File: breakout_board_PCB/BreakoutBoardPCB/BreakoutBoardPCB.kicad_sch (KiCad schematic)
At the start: 16 parts, among them IC1 AD5676BRUZ, IC2 MCP3464T-E_NC, IC3 23K256T-I_SN, IC4 23K256T-I_SN, IC5 23K256T-I_SN, IC6 23K256T-I_SN, IC7 MCP3464T-E_NC, J1 SJ-63062A, J10 Conn_01x27_Female, J11 Conn_01x20_Female, J2 SJ-63062A, J7 Conn_01x06_Female

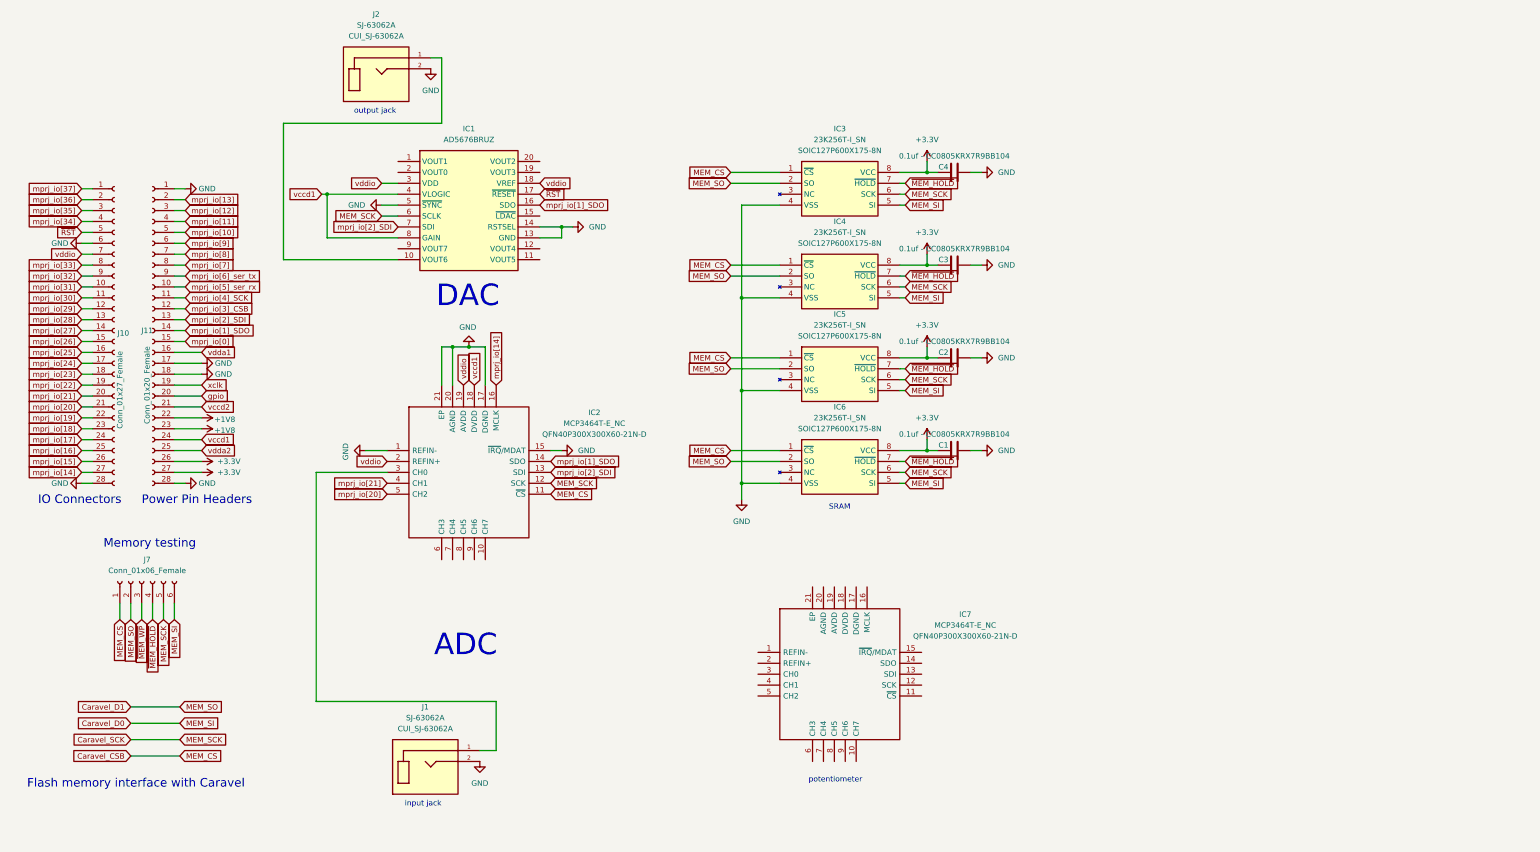
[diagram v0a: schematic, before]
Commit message: update 4/5
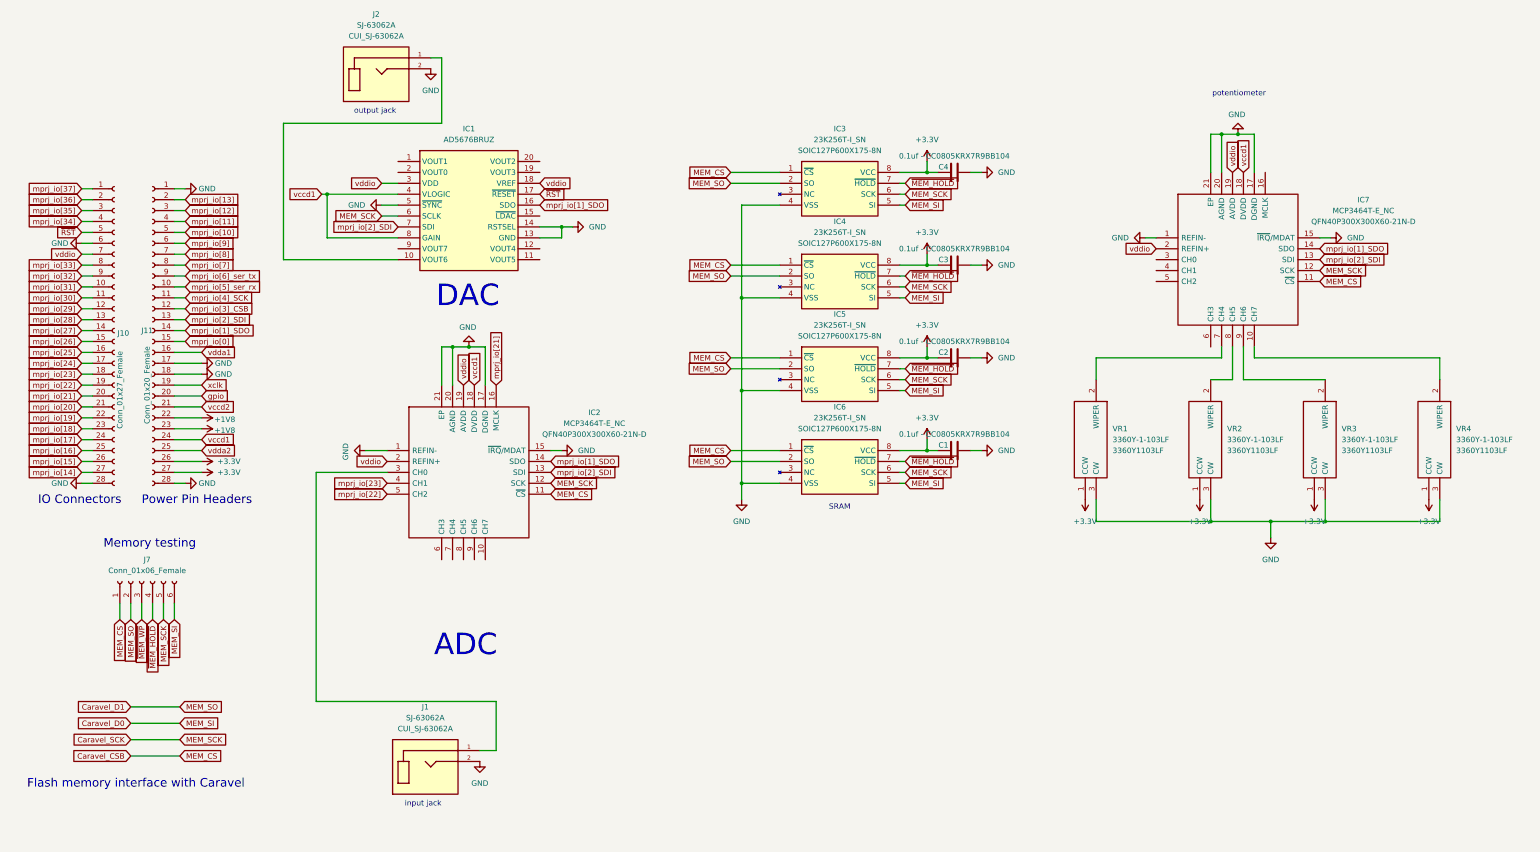
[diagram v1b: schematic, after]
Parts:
- added VR1, VR2, VR3, VR4: 3360Y-1-103LF, 3360Y1103LF, symbol SeniorDesign:3360Y-1-103LF
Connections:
- net +3.3V: now also VR1.1 (CCW), VR2.1 (CCW), VR3.1 (CCW), VR4.1 (CCW)
- net Caravel_CSB: now also IC7.11 (~{CS})
- net Caravel_SCK: now also IC7.12 (SCK)
- net GND: now also IC7.1 (REFIN-), IC7.15 (~{IRQ}/MDAT), IC7.17 (DGND), IC7.20 (AGND), IC7.21 (EP), VR1.3 (CW), VR2.3 (CW), VR3.3 (CW), VR4.3 (CW)
- net mprj_io[14]: no longer IC2.16 (MCLK)
- net mprj_io[1]_SDO: now also IC7.14 (SDO)
- net mprj_io[20]: no longer IC2.5 (CH2)
- net mprj_io[21]: now also IC2.16 (MCLK); no longer IC2.4 (CH1)
- net mprj_io[22]: now also IC2.5 (CH2)
- net mprj_io[23]: now also IC2.4 (CH1)
- net mprj_io[2]_SDI: now also IC7.13 (SDI)
- net vccd1: now also IC7.18 (DVDD)
- net vddio: now also IC7.19 (AVDD), IC7.2 (REFIN+)
- net at IC7.10 (CH7): now also VR4.2 (WIPER)
- net at IC7.7 (CH4): now also VR1.2 (WIPER)
- net at IC7.8 (CH5): now also VR2.2 (WIPER)
- net at IC7.9 (CH6): now also VR3.2 (WIPER)
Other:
- moved on the sheet: IC7

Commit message: last update
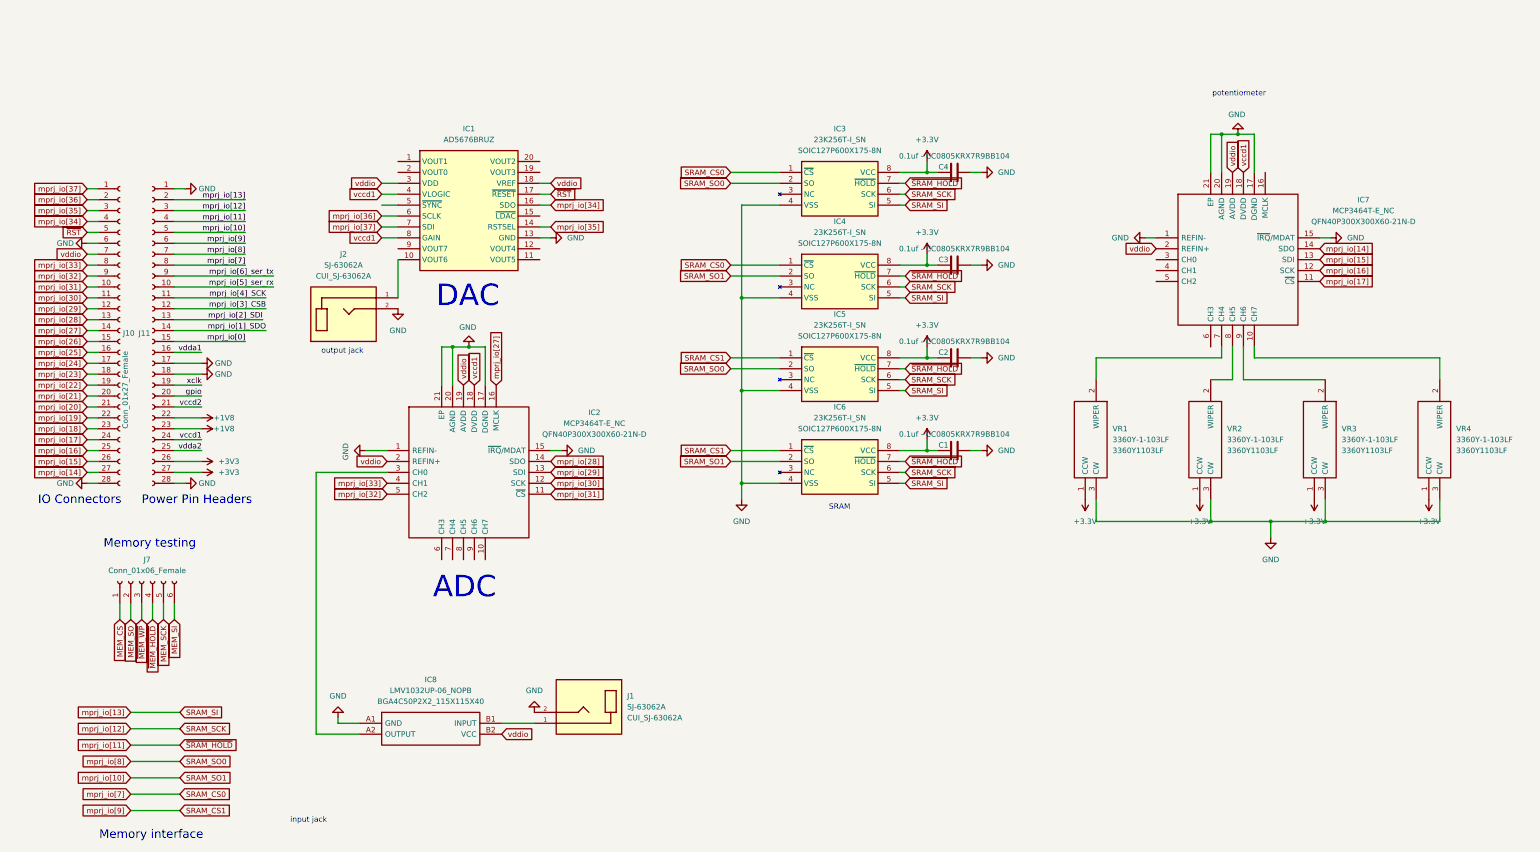
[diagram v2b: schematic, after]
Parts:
- removed J11: Conn_01x20_Female, Connector_PinHeader_2.54mm:PinHeader_1x20_P2.54mm_Vertical, symbol Connector:Conn_01x28_Female
- added IC8: LMV1032UP-06_NOPB, BGA4C50P2X2_115X115X40, symbol SeniorDesign:LMV1032UP-06_NOPB
- added J11: Conn_01x28_Pin, Connector_PinHeader_2.54mm:PinHeader_1x28_P2.54mm_Vertical, symbol Connector:Conn_01x28_Socket
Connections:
- net +1V8: now also J11.22 (Pin_22), J11.23 (Pin_23)
- net GND: now also IC8.A1 (GND), J11.1 (Pin_1), J11.17 (Pin_17), J11.18 (Pin_18), J11.28 (Pin_28); no longer IC1.14 (RSTSEL), IC1.5 (~{SYNC})
- net gpio: now also J11.20 (Pin_20)
- net mprj_io[0]: now also J11.15 (Pin_15)
- net mprj_io[11]: now also IC3.7 (~{HOLD}), IC4.7 (~{HOLD}), IC5.7 (~{HOLD}), IC6.7 (~{HOLD}), J11.4 (Pin_4)
- net mprj_io[14]: now also IC7.14 (SDO)
- net mprj_io[15]: now also IC7.13 (SDI)
- net mprj_io[16]: now also IC7.12 (SCK)
- net mprj_io[17]: now also IC7.11 (~{CS})
- net mprj_io[1]_SDO: now also J11.14 (Pin_14); no longer IC1.16 (SDO), IC2.14 (SDO), IC7.14 (SDO)
- net mprj_io[21]: no longer IC2.16 (MCLK)
- net mprj_io[22]: no longer IC2.5 (CH2)
- net mprj_io[23]: no longer IC2.4 (CH1)
- net mprj_io[27]: now also IC2.16 (MCLK)
- net mprj_io[28]: now also IC2.14 (SDO)
- net mprj_io[29]: now also IC2.13 (SDI)
- net mprj_io[2]_SDI: now also J11.13 (Pin_13); no longer IC1.7 (SDI), IC2.13 (SDI), IC7.13 (SDI)
- net mprj_io[30]: now also IC2.12 (SCK)
- net mprj_io[31]: now also IC2.11 (~{CS})
- net mprj_io[32]: now also IC2.5 (CH2)
- net mprj_io[33]: now also IC2.4 (CH1)
- net mprj_io[34]: now also IC1.16 (SDO)
- net mprj_io[35]: now also IC1.14 (RSTSEL)
- net mprj_io[36]: now also IC1.6 (SCLK)
- net mprj_io[37]: now also IC1.7 (SDI)
- net mprj_io[3]_CSB: now also J11.12 (Pin_12)
- net mprj_io[4]_SCK: now also J11.11 (Pin_11)
- net mprj_io[5]_ser_rx: now also J11.10 (Pin_10)
- net mprj_io[6]_ser_tx: now also J11.9 (Pin_9)
- net vccd1: now also J11.24 (Pin_24)
- net vccd2: now also J11.21 (Pin_21)
- net vdda1: now also J11.16 (Pin_16)
- net vdda2: now also J11.25 (Pin_25)
- net vddio: now also IC8.B2 (VCC)
- net xclk: now also J11.19 (Pin_19)
- net ~{MEM_HOLD}: no longer IC3.7 (~{HOLD}), IC4.7 (~{HOLD}), IC5.7 (~{HOLD}), IC6.7 (~{HOLD})
- net at IC2.3 (CH0): now also IC8.A2 (OUTPUT); no longer J1.1
- removed net Caravel_CSB: IC2.11 (~{CS}), IC3.1 (~{CS}), IC4.1 (~{CS}), IC5.1 (~{CS}), IC6.1 (~{CS}), IC7.11 (~{CS}), J7.1 (Pin_1)
- net Caravel_D0 renamed SRAM_SI
- net SRAM_SI: now also J11.2 (Pin_2); no longer J7.6 (Pin_6)
- removed net Caravel_D1: IC3.2 (SO), IC4.2 (SO), IC5.2 (SO), IC6.2 (SO), J7.2 (Pin_2)
- net Caravel_SCK renamed SRAM_SCK
- net SRAM_SCK: now also J11.3 (Pin_3); no longer IC1.6 (SCLK), IC2.12 (SCK), IC7.12 (SCK), J7.5 (Pin_5)
- new net: IC8.B1 (INPUT), J1.1
- new net +3V3: J11.26 (Pin_26), J11.27 (Pin_27)
- new net MEM_CS: J7.1 (Pin_1)
- new net MEM_SCK: J7.5 (Pin_5)
- new net MEM_SI: J7.6 (Pin_6)
- new net MEM_SO: J7.2 (Pin_2)
- new net SRAM_CS0: IC3.1 (~{CS}), IC4.1 (~{CS}), J11.8 (Pin_8)
- new net SRAM_CS1: IC5.1 (~{CS}), IC6.1 (~{CS}), J11.6 (Pin_6)
- new net SRAM_SO0: IC3.2 (SO), IC5.2 (SO), J11.7 (Pin_7)
- new net SRAM_SO1: IC4.2 (SO), IC6.2 (SO), J11.5 (Pin_5)
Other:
- note added: "Memory interface"
- note removed: "Flash memory interface with Caravel"
- moved on the sheet: J1, J2
